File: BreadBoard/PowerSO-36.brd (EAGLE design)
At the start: 33 x 45.7 mm, 7 parts

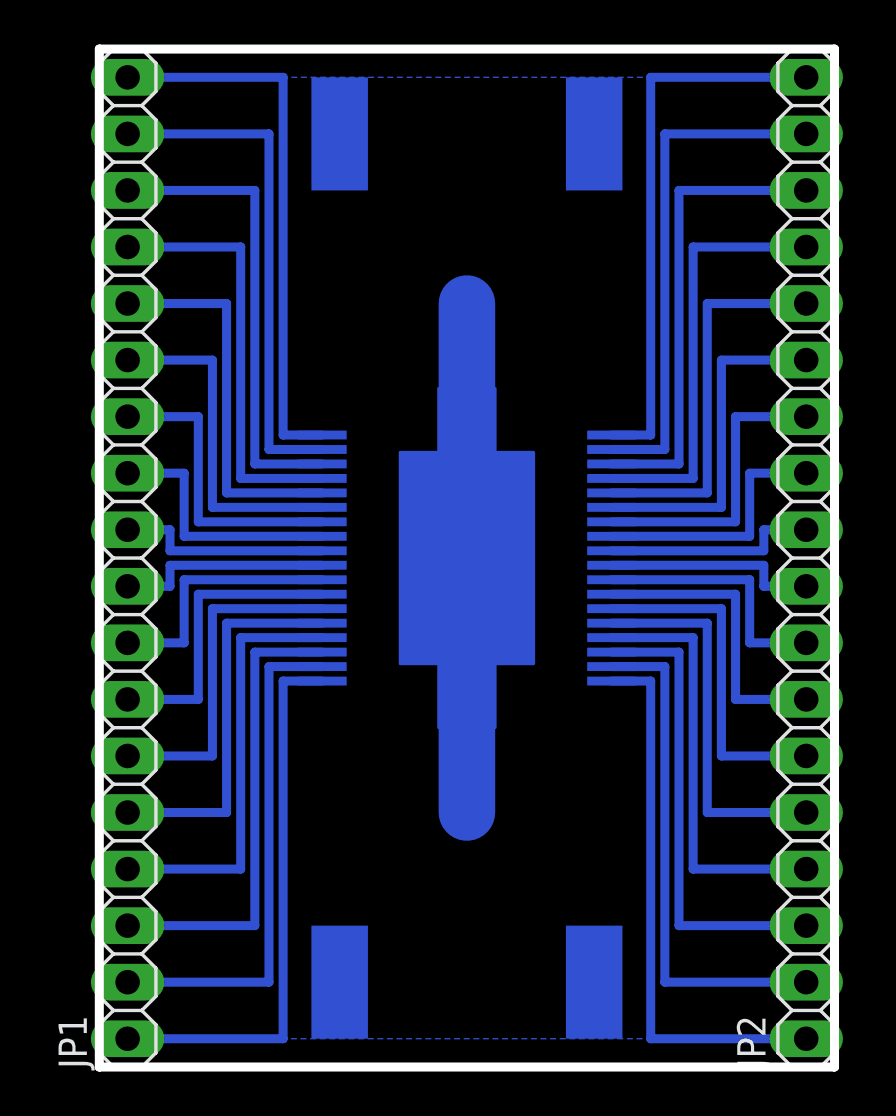
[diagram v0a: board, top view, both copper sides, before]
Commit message: _
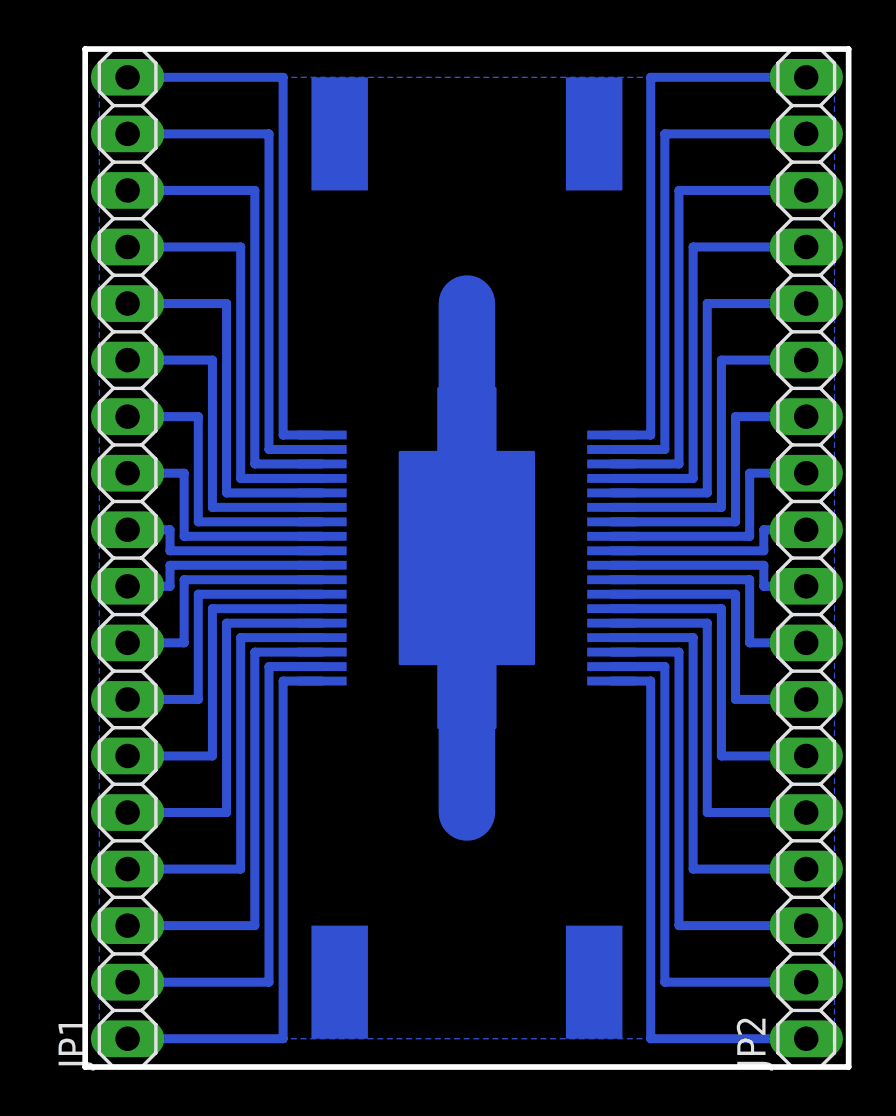
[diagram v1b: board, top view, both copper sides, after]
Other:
- board size 33 x 45.7 mm -> 34.3 x 45.7 mm
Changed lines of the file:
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@@
 <?xml version="1.0" encoding="utf-8"?>
 <!DOCTYPE eagle SYSTEM "eagle.dtd">
-<eagle version="8.0.2">
+<eagle version="8.1.0">
 <drawing>
 <settings>
@@
 <board>
 <plain>
-<wire x1="5.08" y1="46.99" x2="5.08" y2="1.27" width="0.4064" layer="20"/>
-<wire x1="5.08" y1="1.27" x2="38.1" y2="1.27" width="0.4064" layer="20"/>
-<wire x1="38.1" y1="1.27" x2="38.1" y2="46.99" width="0.4064" layer="20"/>
-<wire x1="38.1" y1="46.99" x2="5.08" y2="46.99" width="0.4064" layer="20"/>
+<wire x1="4.445" y1="46.99" x2="4.445" y2="1.27" width="0.254" layer="20"/>
+<wire x1="4.445" y1="1.27" x2="38.735" y2="1.27" width="0.254" layer="20"/>
+<wire x1="38.735" y1="1.27" x2="38.735" y2="46.99" width="0.254" layer="20"/>
+<wire x1="38.735" y1="46.99" x2="4.445" y2="46.99" width="0.254" layer="20"/>
 </plain>
 <attributes>
@@
 <wire x1="21.59" y1="24.13" x2="21.59" y2="12.7" width="2.54" layer="16"/>
 <wire x1="21.59" y1="24.13" x2="21.59" y2="35.56" width="2.54" layer="16"/>
-<polygon width="0.4064" layer="16" isolate="0.8128">
+<polygon width="0.254" layer="16" isolate="0.8128">
 <vertex x="5.08" y="45.72"/>
 <vertex x="38.1" y="45.72"/>
